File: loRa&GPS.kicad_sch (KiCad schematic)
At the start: 23 parts, among them SW3 RESET, SW4 BOOT

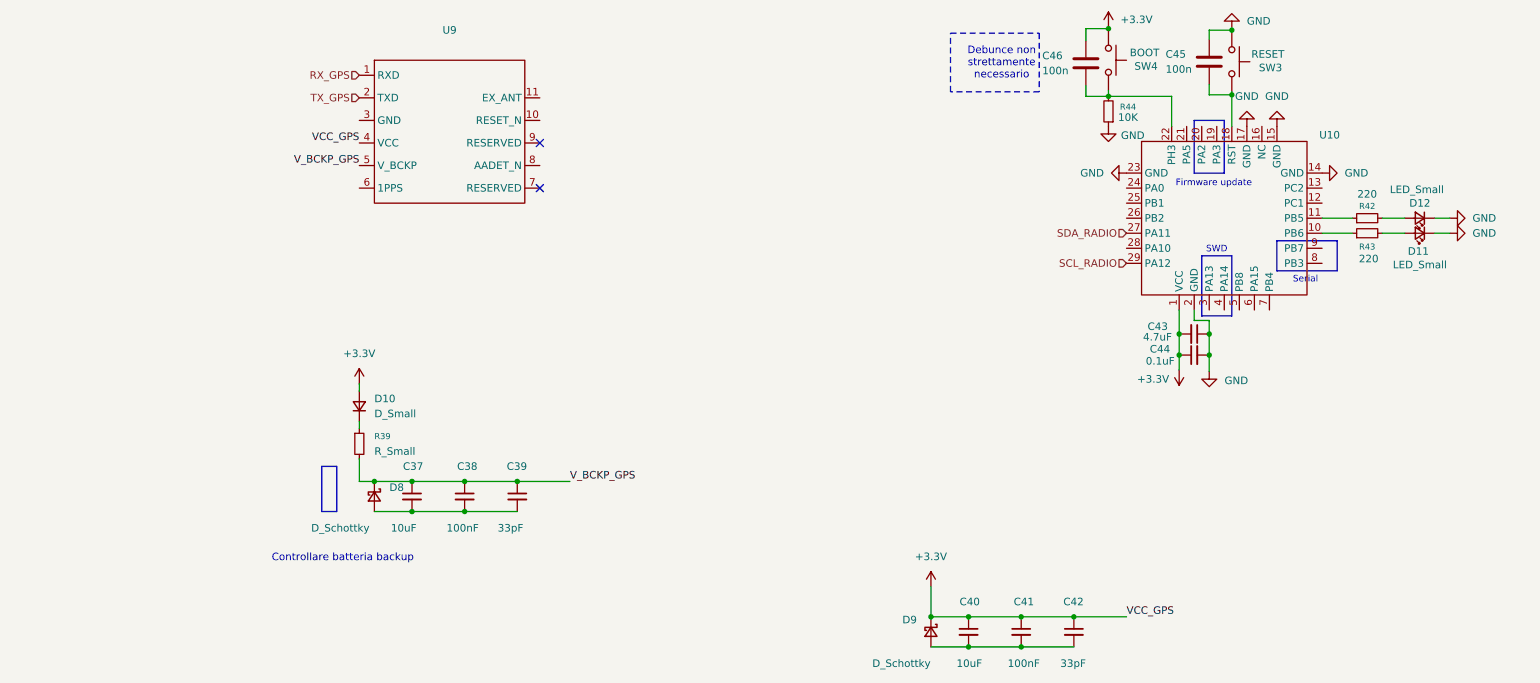
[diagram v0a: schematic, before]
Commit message: Corrections
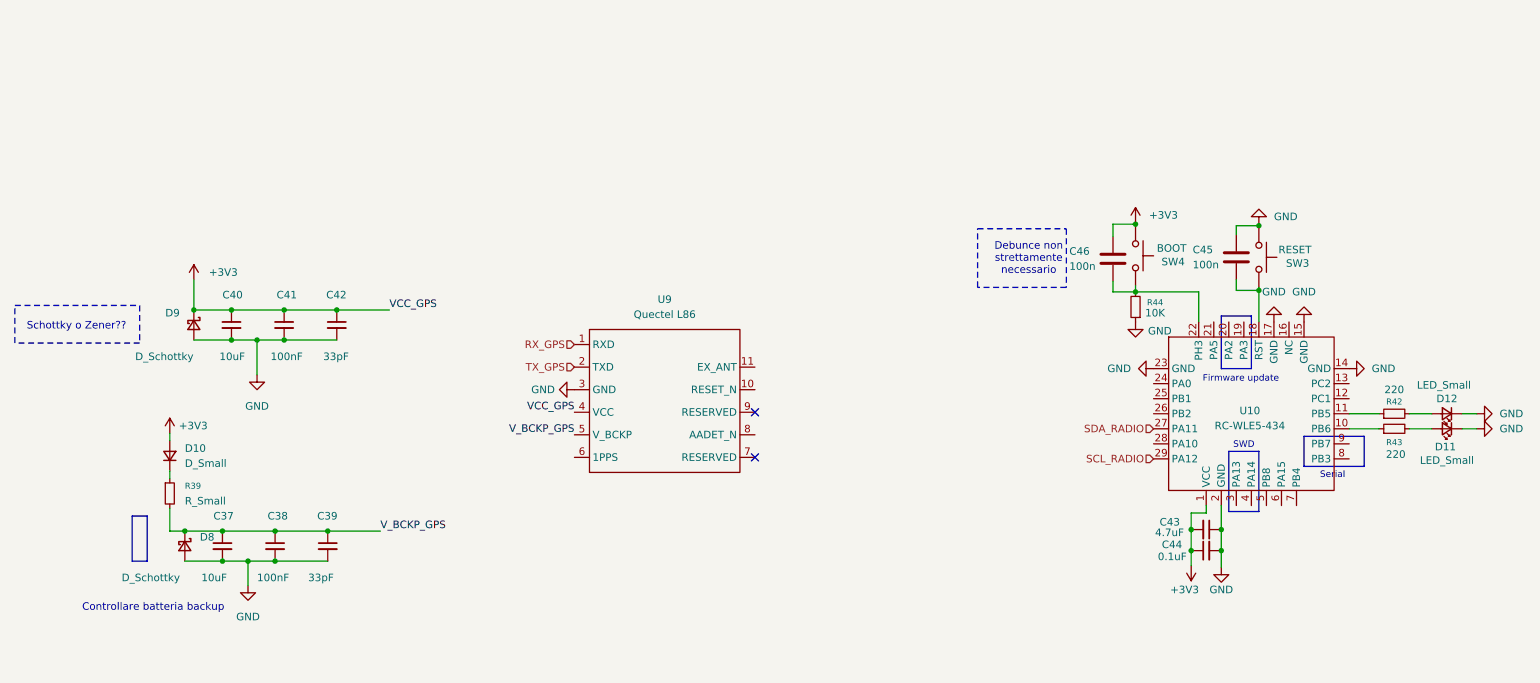
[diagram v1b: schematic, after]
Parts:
- U10: value ~ -> RC-WLE5-434
- U9: value ~ -> Quectel L86
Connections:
- net GND: now also C37.2, C38.2, C39.2, C40.2, C41.2, C42.2, D8.2 (A), D9.2 (A), U9.3 (GND)
- net +3.3V renamed +3V3
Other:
- note added: "Schottky o Zener??"
- moved on the sheet: C37, C38, C39, C40, C41, C42, C43, C44, C45, C46, D10, D11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
